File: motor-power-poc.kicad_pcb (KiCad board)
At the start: 4 copper layers, 150 parts, among them J1 Conn_01x04_Pin, J2 USB_C_Receptacle_USB2.0_14P, J3 Conn_01x02, J4 Conn_02x02_Counter_Clockwise, J5 Conn_02x06_Counter_Clockwise, M1 Motor_Servo, M2 Motor_Servo, M3 DC, Q1 Q_NMOS, Q10 Q_NMOS, Q2 Q_NMOS, Q3 Q_NMOS, Q4 Q_NMOS, Q5 Q_NMOS, Q6 Q_NMOS, Q7 Q_NMOS, Q8 Q_NMOS, Q9 Q_NMOS, SW1 SW_Push, SW2 SW_Push, U1 QRE1113GR, U10 CJ431, U11 DRV8701, U2 QRE1113GR, U3 QRE1113GR, U4 ESP32-S3FH4R2, U5 LM74502, U6 TPS5430DDA, U7 TPS56A37, U8 TPS2121, U9 LDL212PV33R, Y1 48M

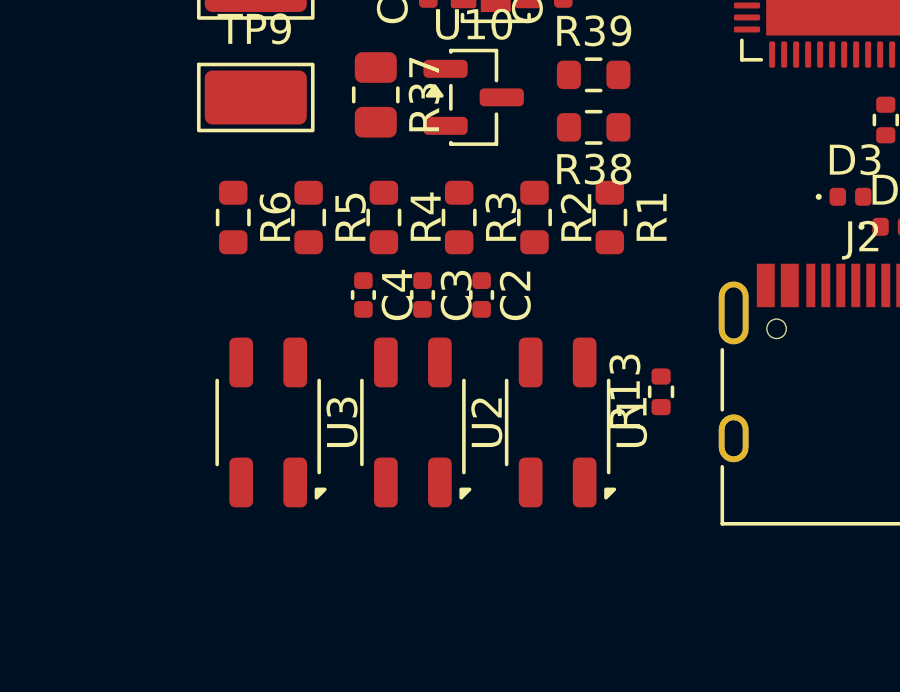
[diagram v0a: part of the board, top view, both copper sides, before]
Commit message: pcb: add QR113 layout
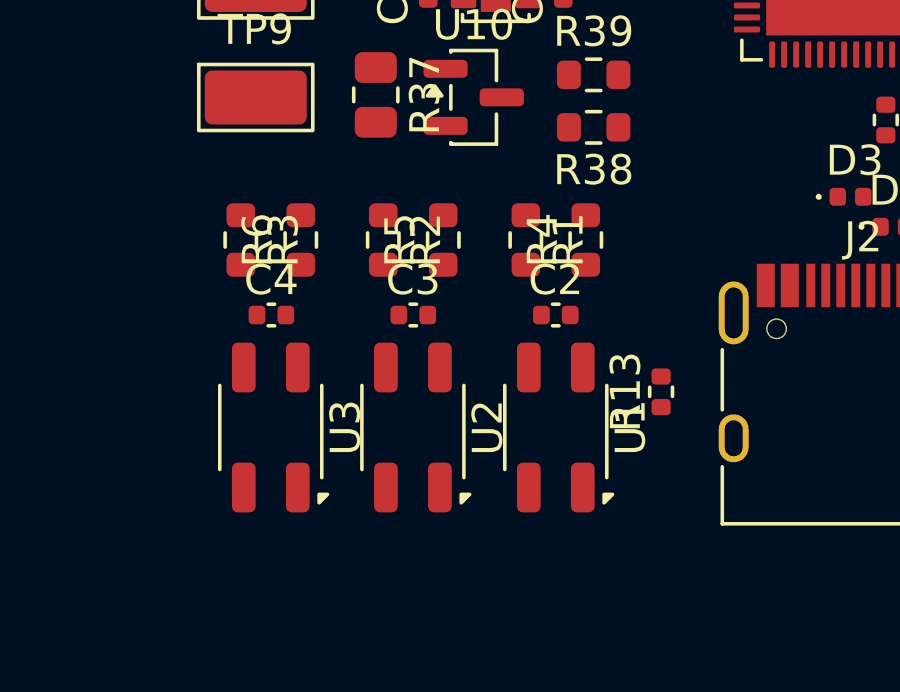
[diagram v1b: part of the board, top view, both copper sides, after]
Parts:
- moved R3 7.32 mm to (113.5, 94.5)
- moved R4 6.77 mm to (125.0, 94.5), turned to 90 degrees
- moved R2 5.10 mm to (118.2, 94.5)
- moved R5 4.55 mm to (120.2, 94.5), turned to 90 degrees
- moved C4 3.14 mm to (114.5, 97.0), turned to 0 degrees
- moved R1 2.90 mm to (123.0, 94.5)
- moved C2 2.56 mm to (124.0, 97.0), turned to 0 degrees
- moved R6 2.37 mm to (115.5, 94.5), turned to 90 degrees
- moved C3 0.73 mm to (119.2, 97.0), turned to 0 degrees
- moved U3 0.19 mm to (114.5, 100.8)
- moved U1 0.18 mm to (124.0, 100.8)
- moved U2 0.17 mm to (119.2, 100.8)
